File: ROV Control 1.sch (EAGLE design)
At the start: 6 parts, among them J4 RASPBERRYPI-40-PIN-GPIO_PTH, U1 ARDUINOR3-BPLACE, X1 S4B-ZR

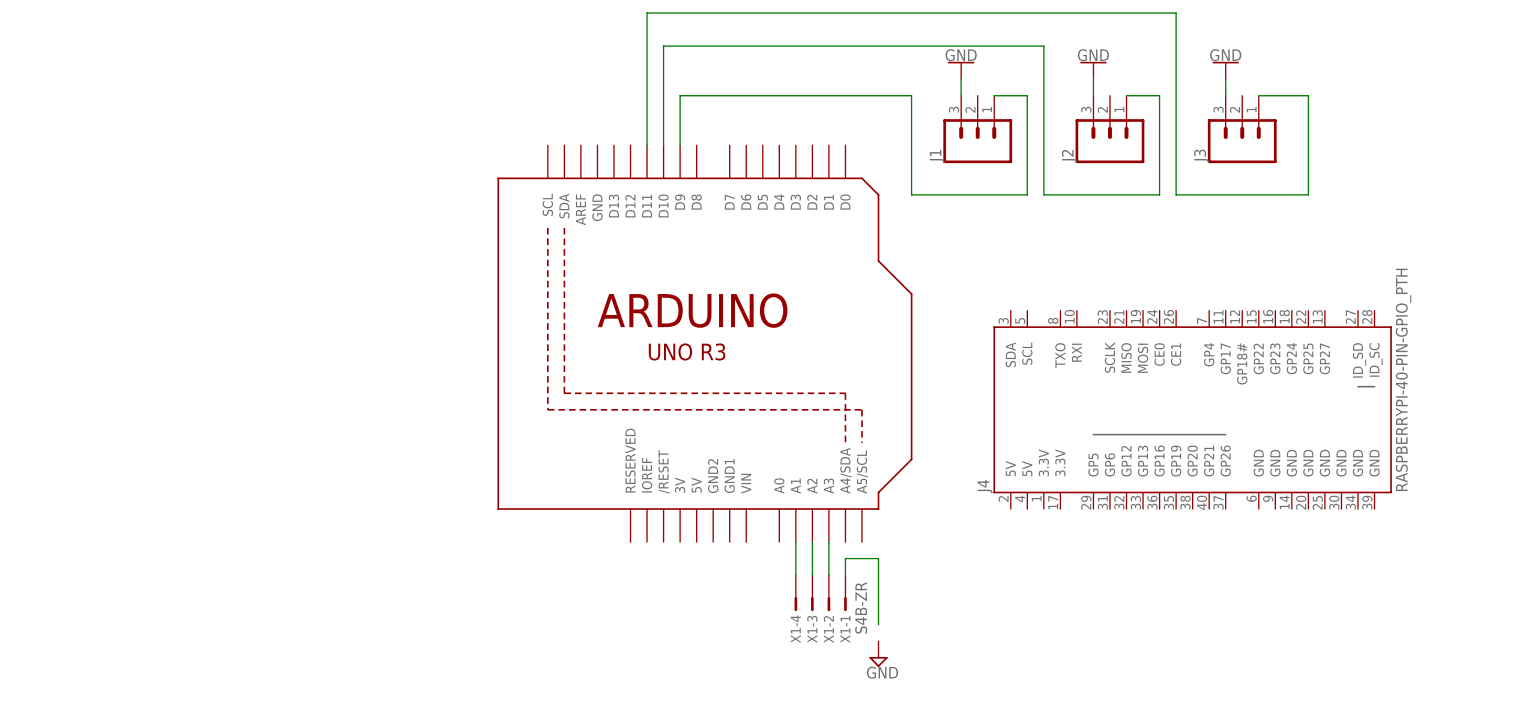
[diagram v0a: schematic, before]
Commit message: Add files via upload
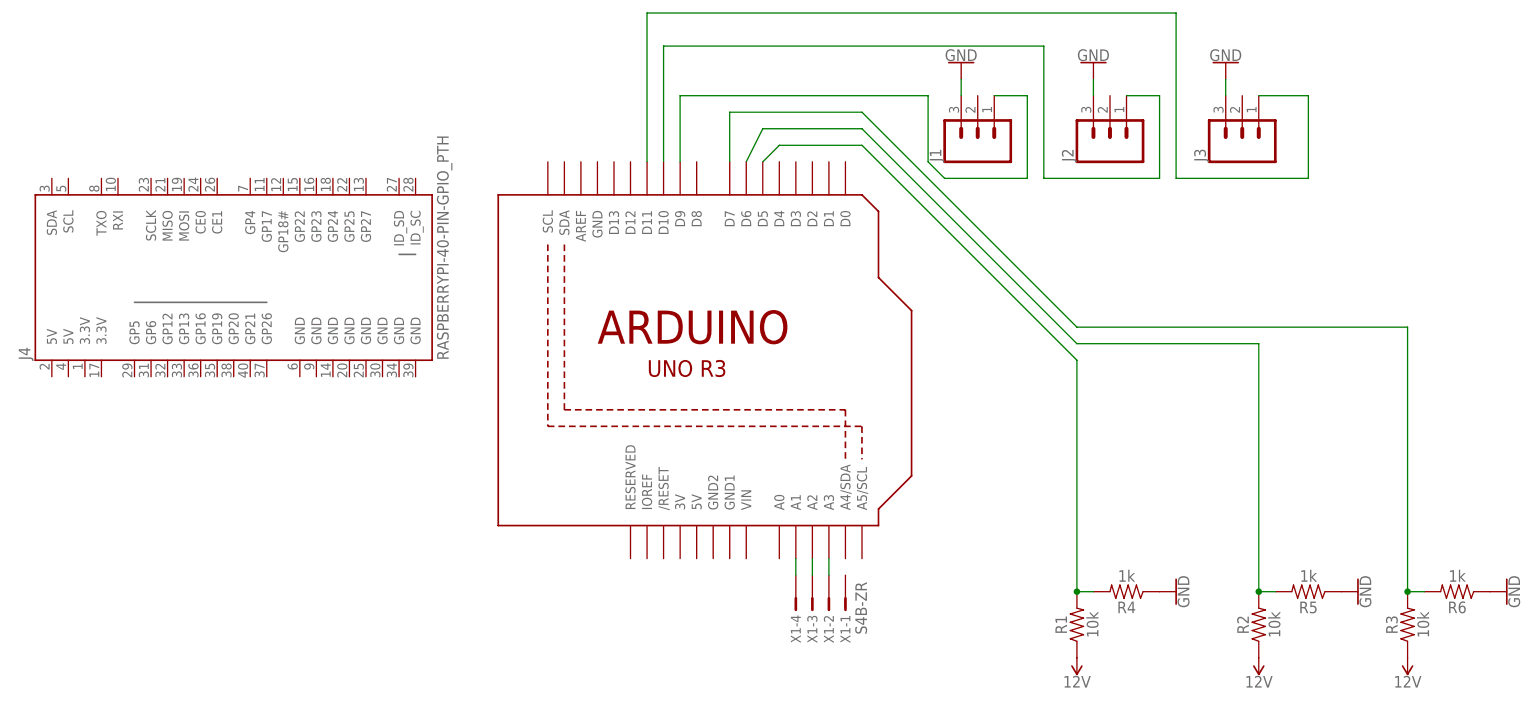
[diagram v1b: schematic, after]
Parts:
- added R1, R2, R3: 10k, SparkFun-Resistors:10KOHM-0603-1/10W-1%
- added R4, R5, R6: 1k, SparkFun-Resistors:1KOHM-0603-1/10W-1%
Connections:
- new net 12V: R1.1, R2.1, R3.1
- new net N$10: R3.2, R6.2, U1.D7
- new net N$9: R2.2, R5.2, U1.D6
- net GND: now also R4.1, R5.1, R6.1
- net N$7: now also R1.2, R4.2, U1.D5; no longer X1-1.1
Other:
- moved on the sheet: J4
